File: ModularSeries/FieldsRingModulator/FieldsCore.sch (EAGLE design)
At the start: 37 parts

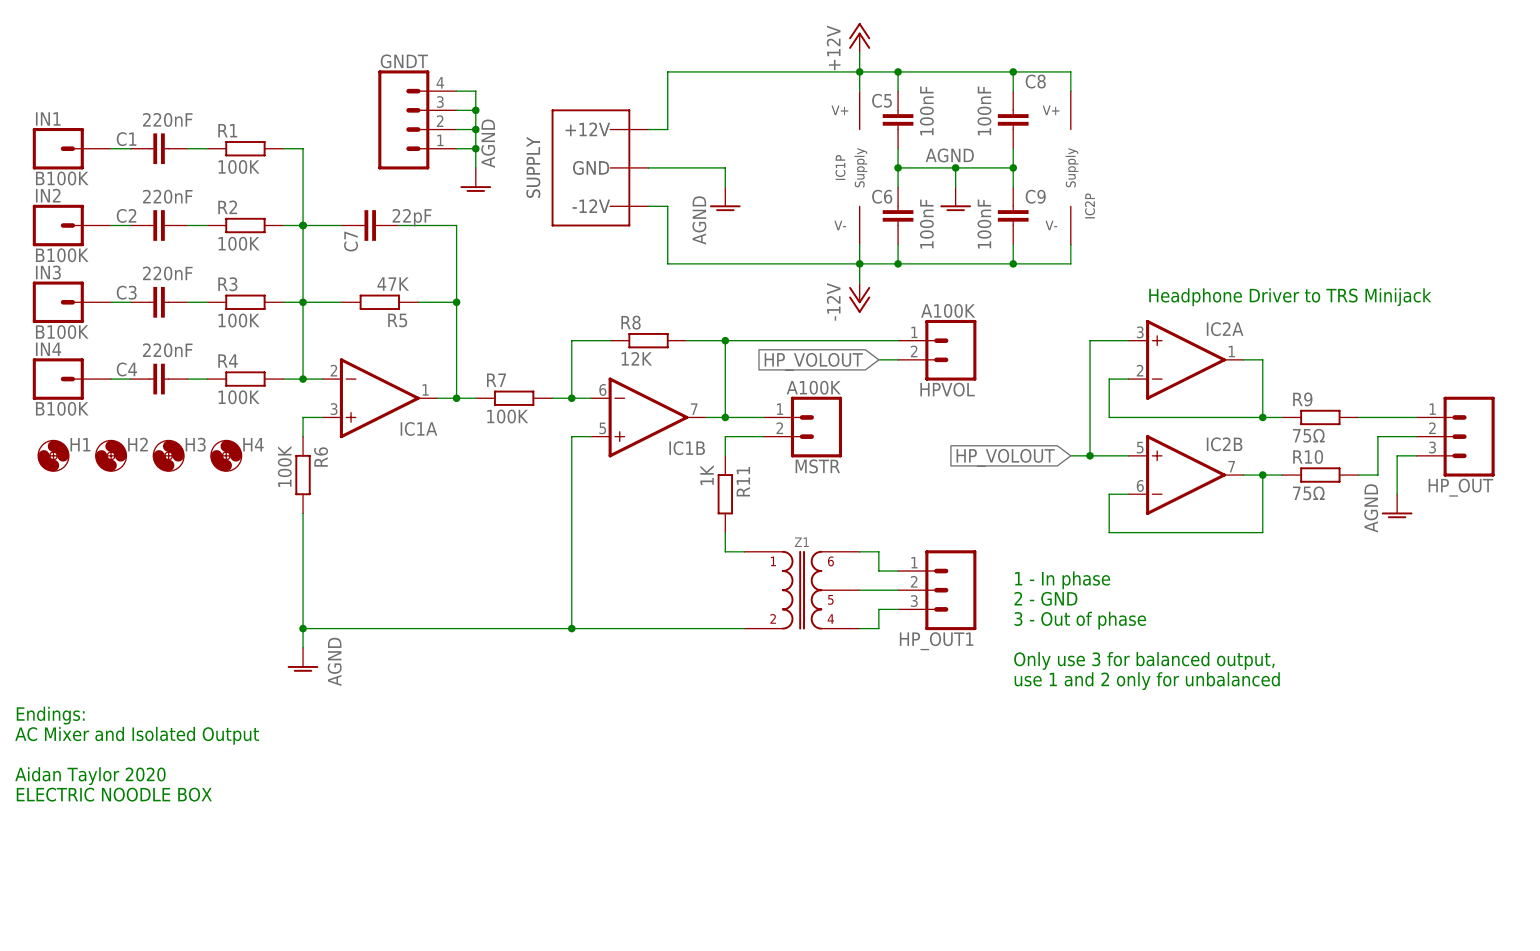
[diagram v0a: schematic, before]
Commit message: Fields added and various updates to designs
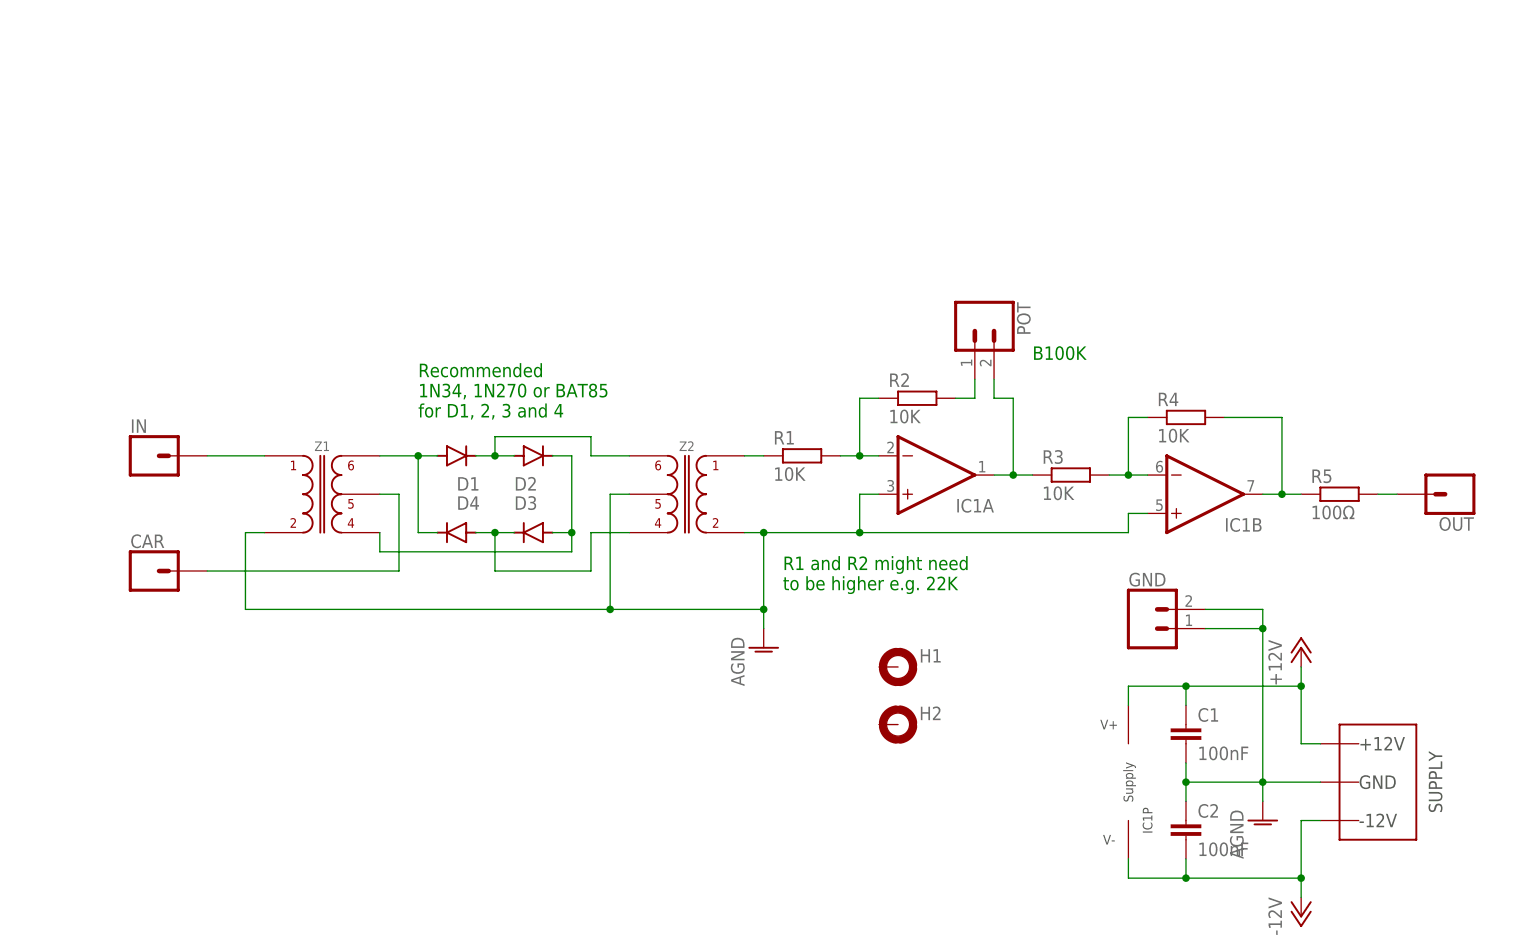
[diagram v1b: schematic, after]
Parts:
- removed C3, C4: 220nF, rcl:C-EU050-025X075
- removed C5, C6, C8, C9: 100nF, rcl:C-EU050-025X075
- removed C7: 22pF, rcl:C-EU050-025X075
- removed GNDT: 4XWIREPAD, ElectricNoodleBox:4XWIREPAD
- removed H3, H4: MOUNT-HOLE3.2, holes:MOUNT-HOLE3.2
- removed HPVOL, MSTR: A100K, ElectricNoodleBox:2XWIREPAD
- removed HP_OUT, HP_OUT1: 3XWIREPAD, ElectricNoodleBox:3XWIREPAD
- removed IC2: (no value), ElectricNoodleBox:TL0X2DIL
- removed IN1, IN2, IN3, IN4: B100K, ElectricNoodleBox:1XWIREPAD
- removed R10, R9: 75Ω, rcl:R-EU_0207/10
- removed R11: 1K, rcl:R-EU_0207/10
- removed R6, R7: 100K, rcl:R-EU_0207/10
- removed R8: 12K, rcl:R-EU_0207/10
- added CAR, IN, OUT: 1XWIREPAD, ElectricNoodleBox:1XWIREPAD
- added D1, D2, D3, D4: (no value), diode:DIODE-DO35-10
- added GND, POT: 2XWIREPAD, ElectricNoodleBox:2XWIREPAD
- added Z2: (no value), ElectricNoodleBox:Z1604_AUDIO_TRANSFORMER
- C1, C2: value 220nF -> 100nF
- H1, H2: value MOUNT-HOLE3.2 -> MOUNT-PAD-ROUND3.2; device holes:MOUNT-HOLE3.2 -> holes:MOUNT-PAD-ROUND3.2
- R1, R2, R3, R4: value 100K -> 10K
- R5: value 47K -> 100Ω
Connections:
- removed net HP_VOLOUT: HPVOL.2, IC2A.+IN, IC2B.+IN
- removed net N$15: HP_OUT1.1, Z1.6
- removed net N$16: HP_OUT1.2, Z1.5
- removed net N$17: HP_OUT1.3, Z1.4
- removed net N$18: IC2A.-IN, IC2A.OUT, R9.1
- removed net N$19: HP_OUT.1, R9.2
- removed net N$20: IC2B.-IN, IC2B.OUT, R10.1
- removed net N$21: HP_OUT.2, R10.2
- removed net N$22: R11.2, Z1.1
- removed net N$9: C2.2, R2.1
- net +12V: now also C1.1; no longer C5.1, C8.1, IC2P.V+
- net -12V: now also C2.2; no longer C6.2, C9.2, IC2P.V-
- net AGND: now also C1.2, C2.1, GND.1, GND.2, IC1A.+IN, Z2.3, Z2.5; no longer C5.2, C6.1, C8.2, C9.1, GNDT.1, GNDT.2, GNDT.3, GNDT.4, HP_OUT.3, R6.2
- net N$1: now also D1.A, D4.C, Z1.6; no longer C4.1, IN4.1
- net N$10: now also POT.1, R2.2; no longer C3.2, R3.1
- net N$11: now also IC1A.OUT, POT.2, R3.1; no longer C4.2, R4.1
- net N$12: now also IC1B.-IN, R3.2, R4.1; no longer C2.1, IN2.1
- net N$13: now also IC1B.OUT, R4.2, R5.1; no longer C1.1, IN1.1
- net N$14: now also OUT.1, R5.2; no longer MSTR.2, R11.1
- net N$2: now also D1.C, D2.A, Z2.6; no longer C7.1, IC1A.-IN, R1.2, R2.2, R3.2, R4.2, R5.2
- net N$3: now also D2.C, D3.A, Z1.4; no longer C7.2, IC1A.OUT, R5.1, R7.1
- net N$4: now also D3.C, D4.A, Z2.4; no longer IC1B.-IN, R7.2, R8.1
- net N$5: now also CAR.1, Z1.5; no longer HPVOL.1, IC1B.OUT, MSTR.1, R8.2
- net N$6: now also R1.1, Z2.1; no longer C3.1, IN3.1
- net N$7: now also IC1A.-IN, R1.2, R2.1; no longer IC1A.+IN, R6.1
- net N$8: now also IN.1, Z1.1; no longer C1.2, R1.1
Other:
- note added: "B100K"
- note added: "R1 and R2 might need to be higher e.g. 22K"
- note added: "Recommended 1N34, 1N270 or BAT85 for D1, 2, 3 and 4"
- note removed: "1 - In phase 2 - GND 3 - Out of phase Only use 3 for balanced output, use 1 and 2 only for unbalanced"
- note removed: "Endings: AC Mixer and Isolated Output Aidan Taylor 2020 ELECTRIC NOODLE BOX"
- note removed: "Headphone Driver to TRS Minijack"
- moved on the sheet: C1, C2, H1, H2, IC1A, IC1B, IC1P, R1, R2, R3, R4, R5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
